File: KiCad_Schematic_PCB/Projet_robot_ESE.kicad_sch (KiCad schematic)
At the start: 0 parts

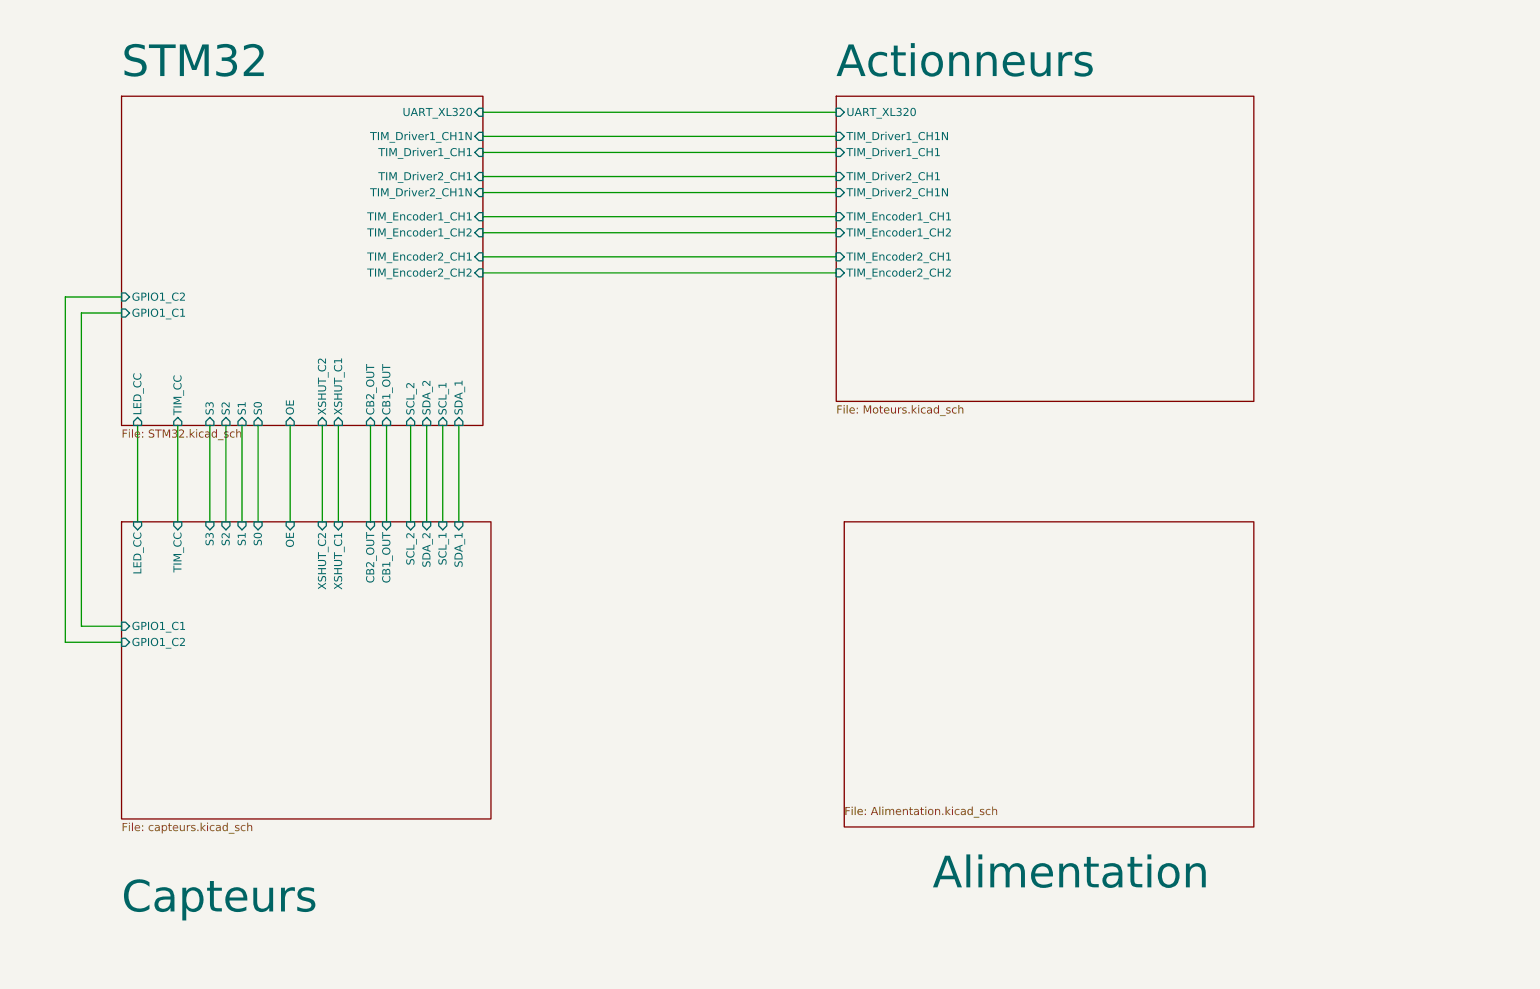
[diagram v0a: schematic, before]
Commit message: Schematic_KiCad_v2
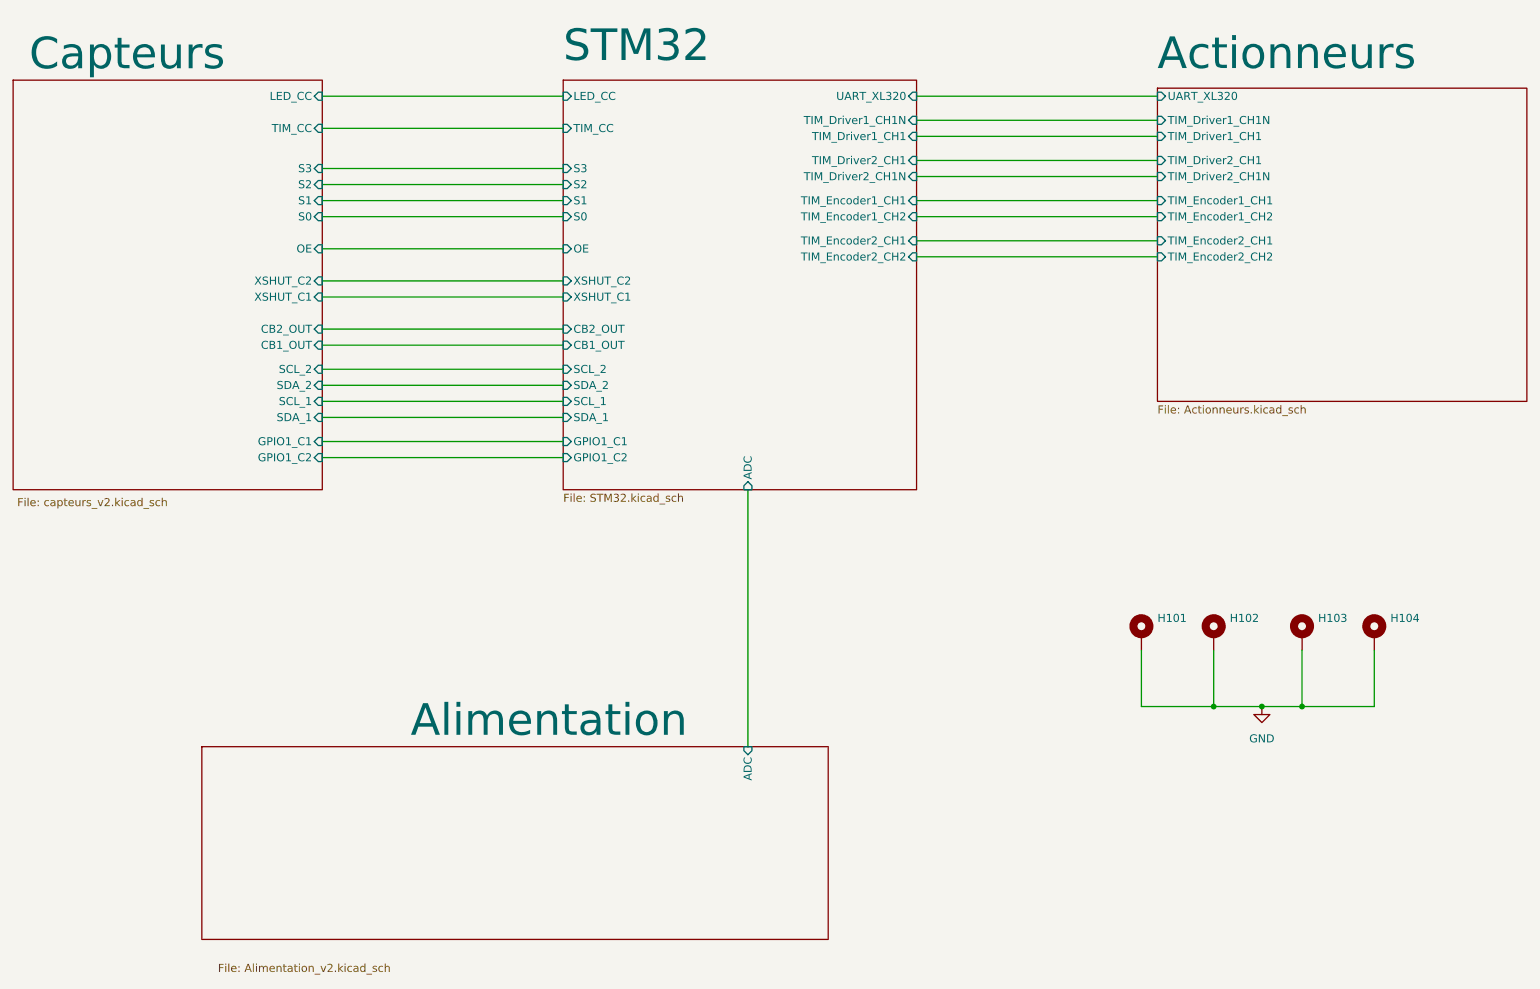
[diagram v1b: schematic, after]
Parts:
- added H101, H102, H103, H104: MountingHole_Pad, MountingHole:MountingHole_3.2mm_M3_Pad_Via, symbol Mechanical:MountingHole_Pad
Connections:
- new net GND: H101.1, H102.1, H103.1, H104.1
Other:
- sheet Actionneurs: file Moteurs.kicad_sch -> Actionneurs.kicad_sch
- sheet Alimentation: file Alimentation.kicad_sch -> Alimentation_v2.kicad_sch
- sheet Alimentation ports: added ADC; removed none
- sheet Capteurs: file capteurs.kicad_sch -> capteurs_v2.kicad_sch
- sheet STM32 ports: added ADC; removed none
